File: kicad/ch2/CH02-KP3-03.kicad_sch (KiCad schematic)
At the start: 5 parts

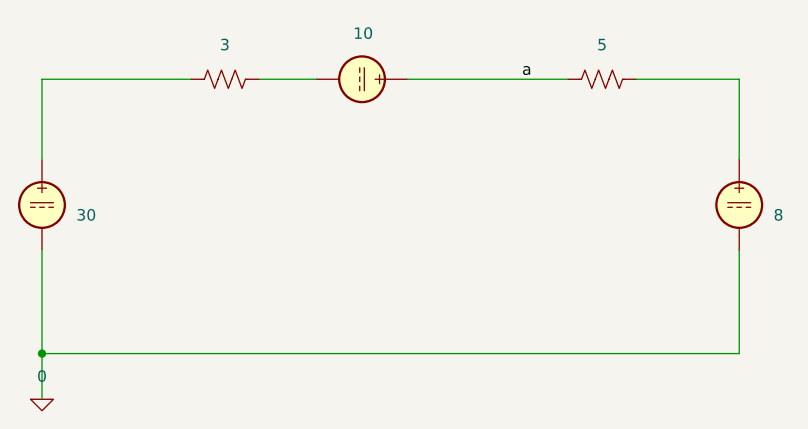
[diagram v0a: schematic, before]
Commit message: regular
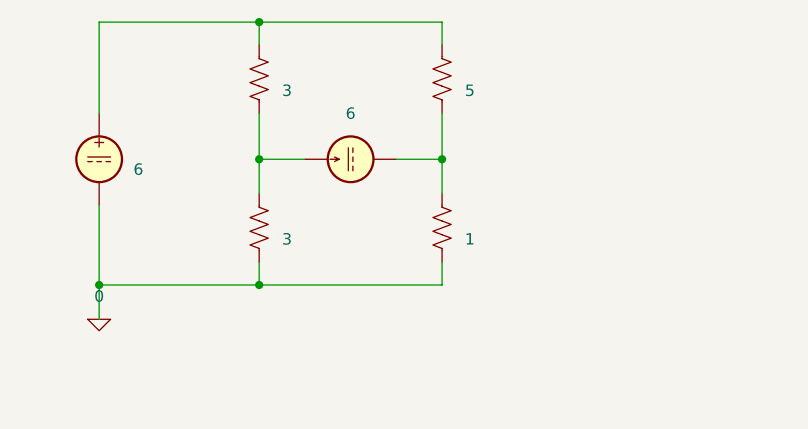
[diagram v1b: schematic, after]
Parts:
- removed R4: 3, symbol Device:R_US
- removed R5: 5, symbol Device:R_US
- removed V3: 30, symbol Simulation_SPICE:VDC
- removed V4: 10, symbol Simulation_SPICE:VDC
- removed V5: 8, symbol Simulation_SPICE:VDC
- added I2: 6, symbol Simulation_SPICE:IDC
- added R10, R12: 3, symbol Device:R_US
- added R11: 5, symbol Device:R_US
- added R13: 1, symbol Device:R_US
- added V7: 6, symbol Simulation_SPICE:VDC
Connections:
- net 0: now also R12.2, R13.2, V7.2
- new net: I2.1, R10.2, R12.1
- new net: I2.2, R11.2, R13.1
- new net: R10.1, R11.1, V7.1
